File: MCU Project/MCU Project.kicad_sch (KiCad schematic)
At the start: 2 parts, among them J1 CONBNC001

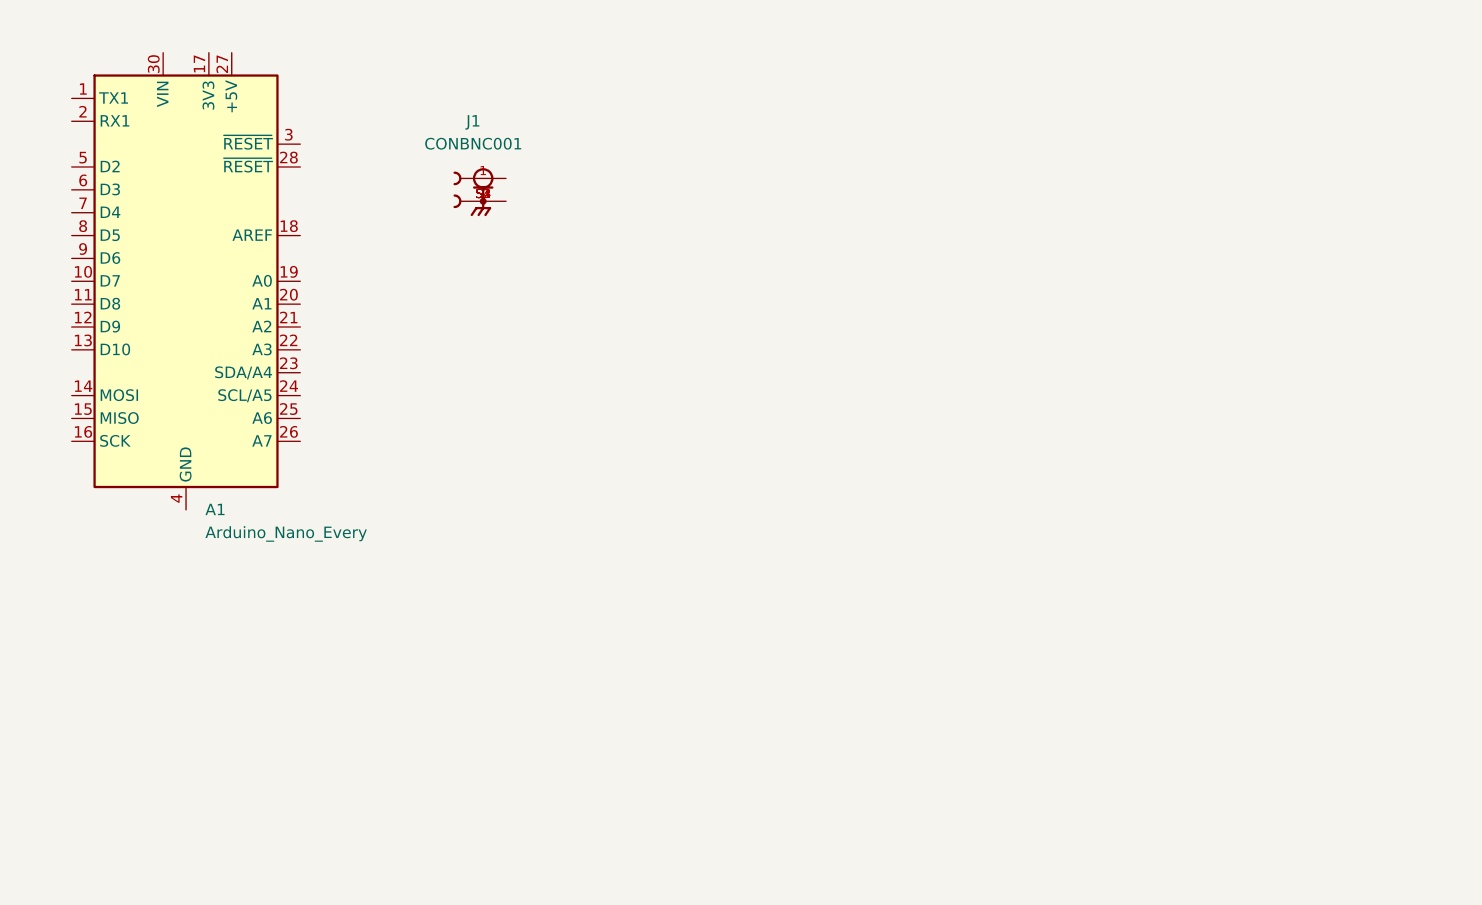
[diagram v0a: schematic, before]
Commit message: Do work
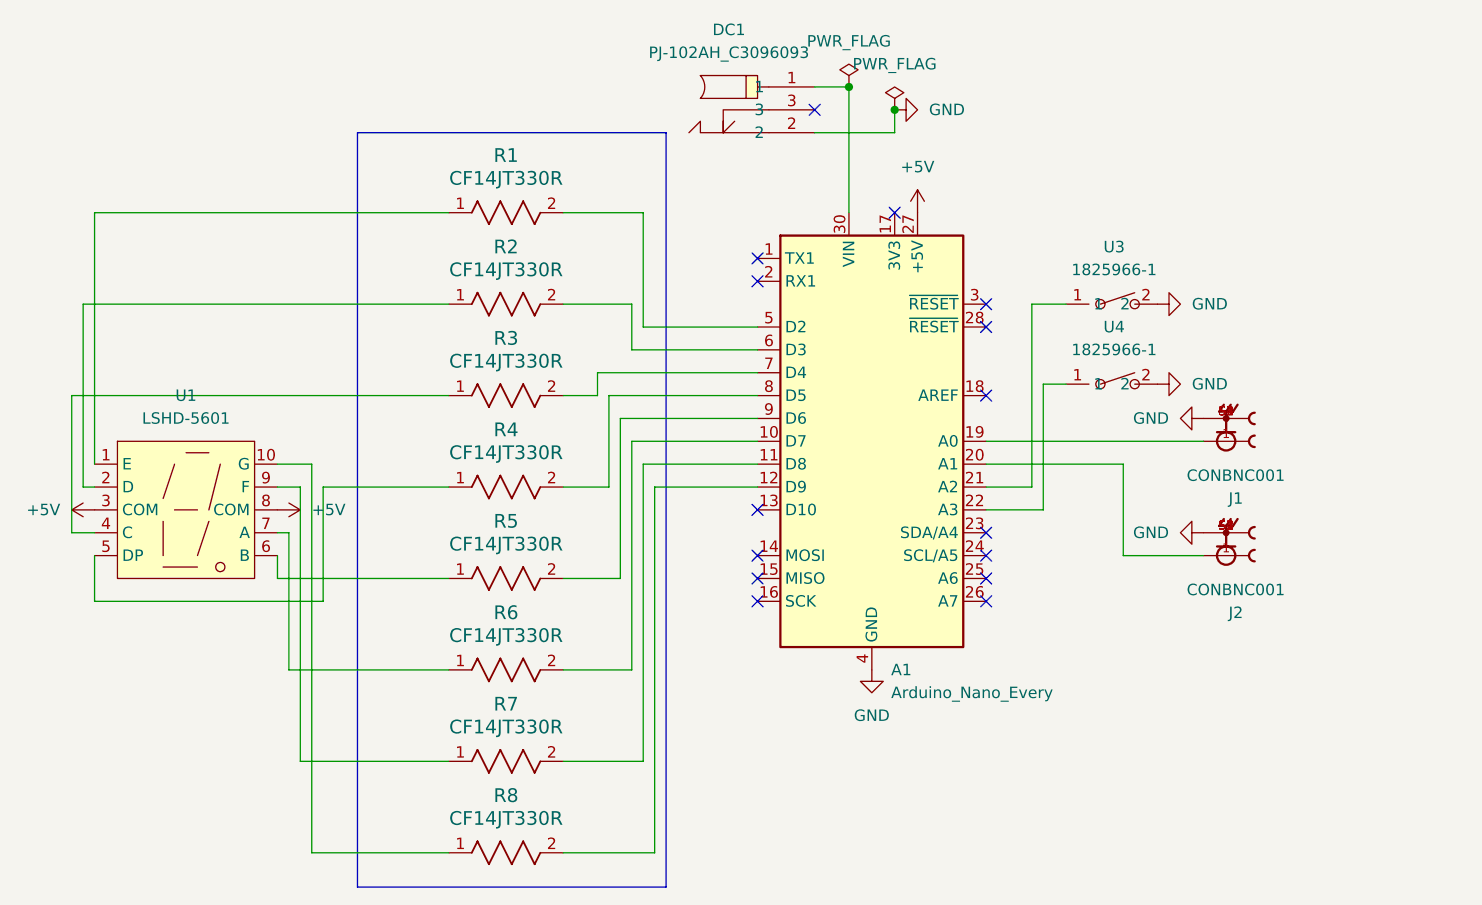
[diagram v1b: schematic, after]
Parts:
- added DC1: PJ-102AH_C3096093, EasyEDA:DC-IN-TH_PJ-102AH, symbol EasyEDA:PJ-102AH_C3096093
- added J2: CONBNC001, Snapeda:LINX_CONBNC001, symbol Snapeda:CONBNC001
- added R1, R2, R3, R4, R5, R6, R7, R8: CF14JT330R, Snapeda:STA_CF14_STP, symbol Snapeda:CF14JT330R
- added U1: LSHD-5601, EasyEDA:LED-SEG-TH_10P-L17.1-W12.4-P2.54-D0.3-LS15.24, symbol EasyEDA:LSHD-5601
- added U3, U4: 1825966-1, EasyEDA:SW-TH_L6.0-W3.6-P6.50, symbol EasyEDA:1825966-1
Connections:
- net at J1.1: now also A1.19 (A0)
- net GND: now reaches J1.S1, J1.S2, J1.S3, J1.S4
- net GND: now also A1.29 (GND), A1.4 (GND), DC1.2, J2.S1, J2.S2, J2.S3, J2.S4, U3.2, U4.2
- net at A1.10 (D7): now also R6.2
- net at A1.11 (D8): now also R7.2
- net at A1.12 (D9): now also R8.2
- net at A1.20 (A1): now also J2.1
- net at A1.21 (A2): now also U3.1
- net at A1.22 (A3): now also U4.1
- net +5V: now reaches A1.27 (+5V)
- net +5V: now also U1.3 (COM), U1.8 (COM)
- net at A1.30 (VIN): now also DC1.1
- net at A1.5 (D2): now also R1.2
- net at A1.6 (D3): now also R2.2
- net at A1.7 (D4): now also R3.2
- net at A1.8 (D5): now also R4.2
- net at A1.9 (D6): now also R5.2
- new net: R7.1, U1.9 (F)
- new net: R1.1, U1.1 (E)
- new net: R8.1, U1.10 (G)
- new net: R4.1, U1.5 (DP)
- new net: R3.1, U1.4 (C)
- new net: R2.1, U1.2 (D)
- new net: R5.1, U1.6 (B)
- new net: R6.1, U1.7 (A)
- no-connect marks 0 -> 15
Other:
- moved on the sheet: A1, J1

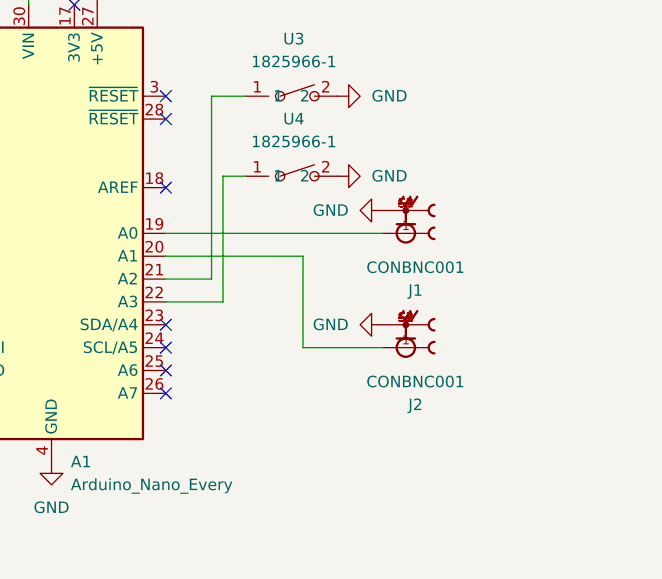
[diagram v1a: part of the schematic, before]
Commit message: Do something
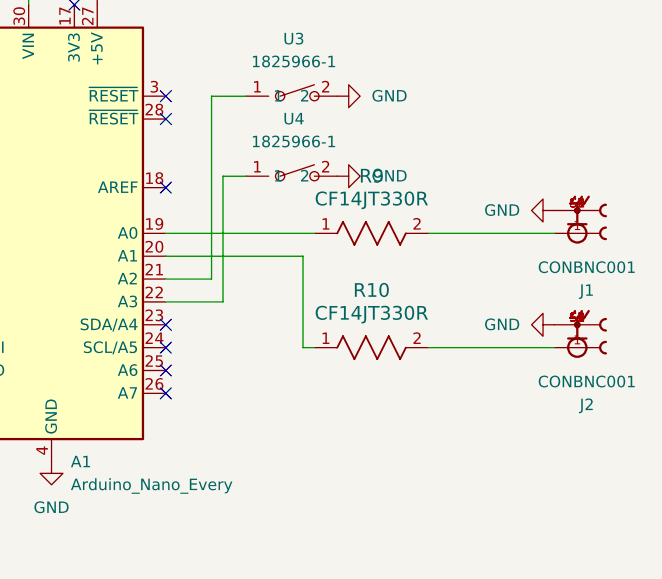
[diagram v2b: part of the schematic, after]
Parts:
- added R10, R9: CF14JT330R, Snapeda:STA_CF14_STP, symbol Snapeda:CF14JT330R
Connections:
- net at J2.1: now also R10.2; no longer A1.20 (A1)
- net at A1.19 (A0): now also R9.1; no longer J1.1
- new net: J1.1, R9.2
- new net: A1.20 (A1), R10.1
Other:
- moved on the sheet: J1, J2
